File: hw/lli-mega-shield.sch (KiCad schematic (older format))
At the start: 6 parts

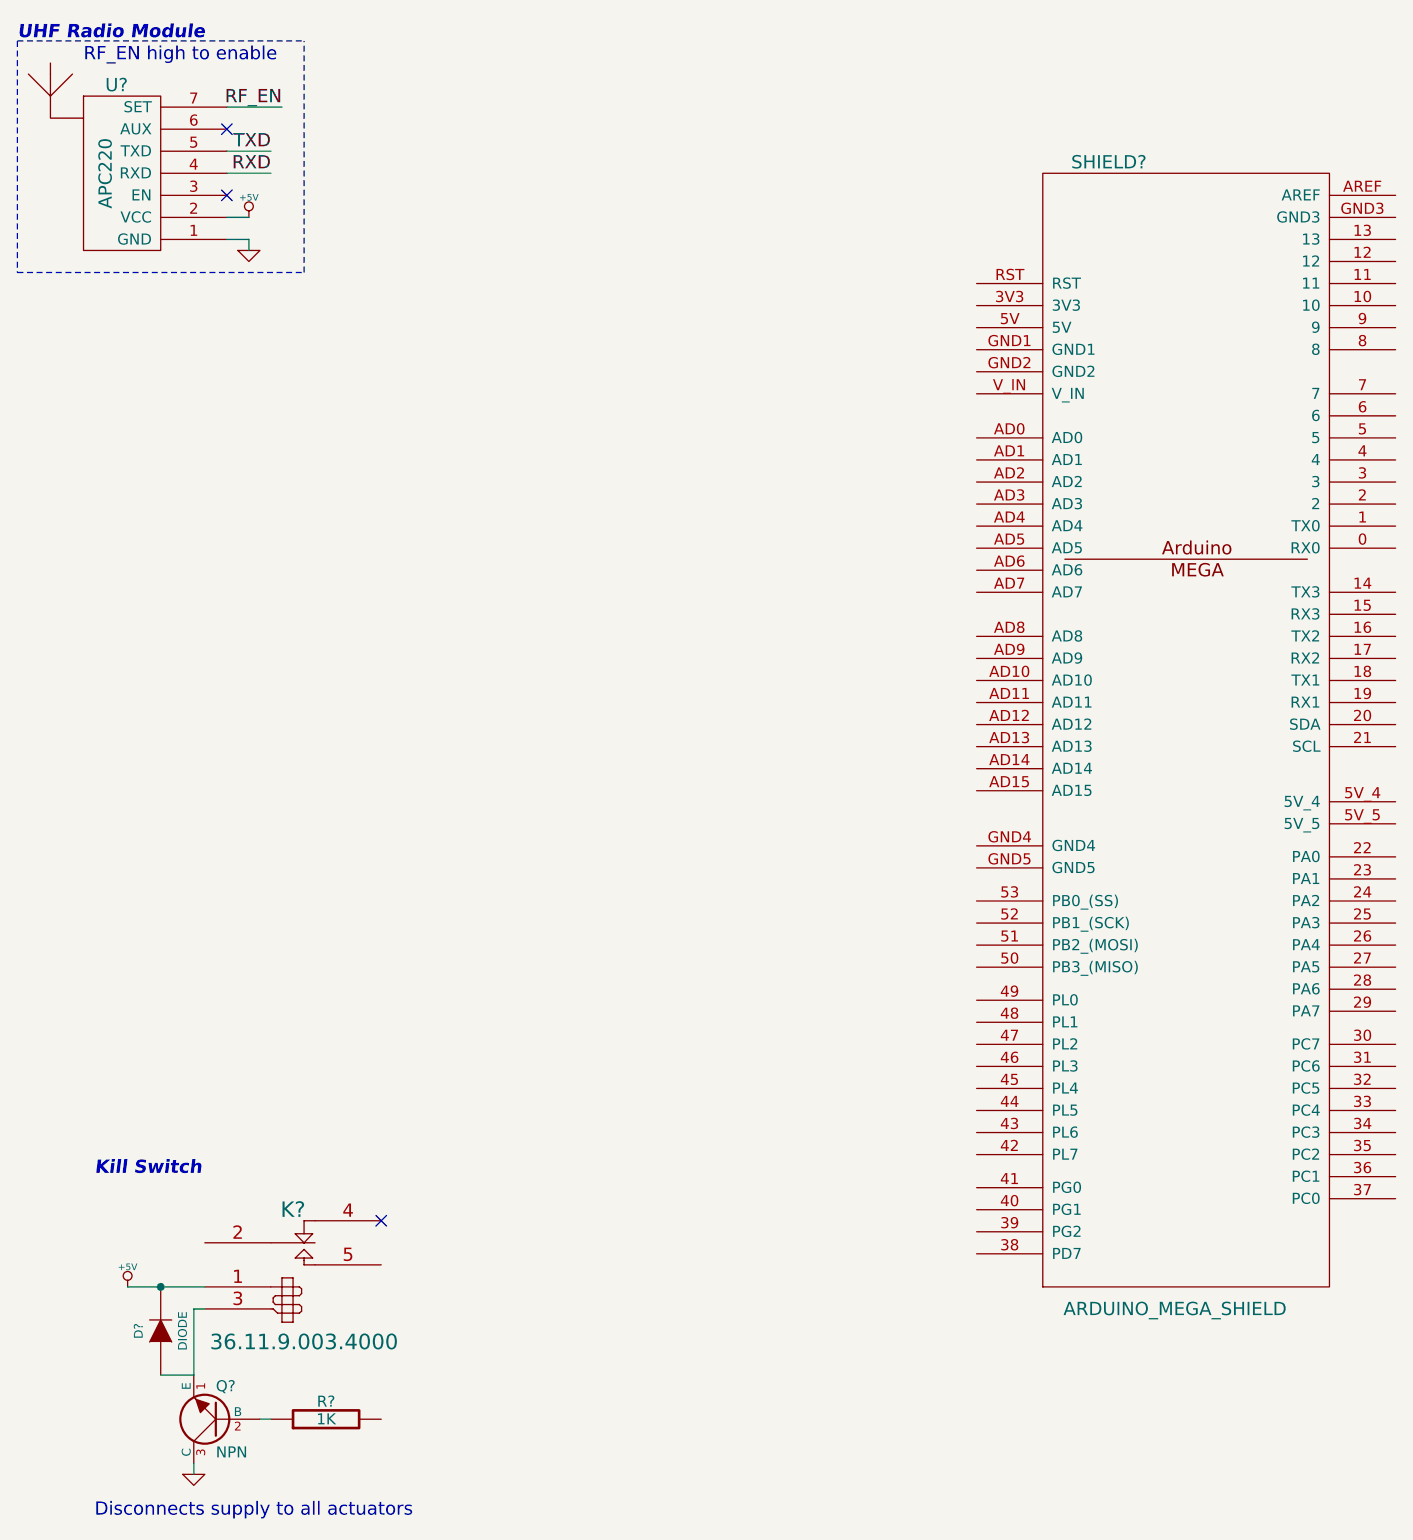
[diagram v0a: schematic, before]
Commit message: Some schematics
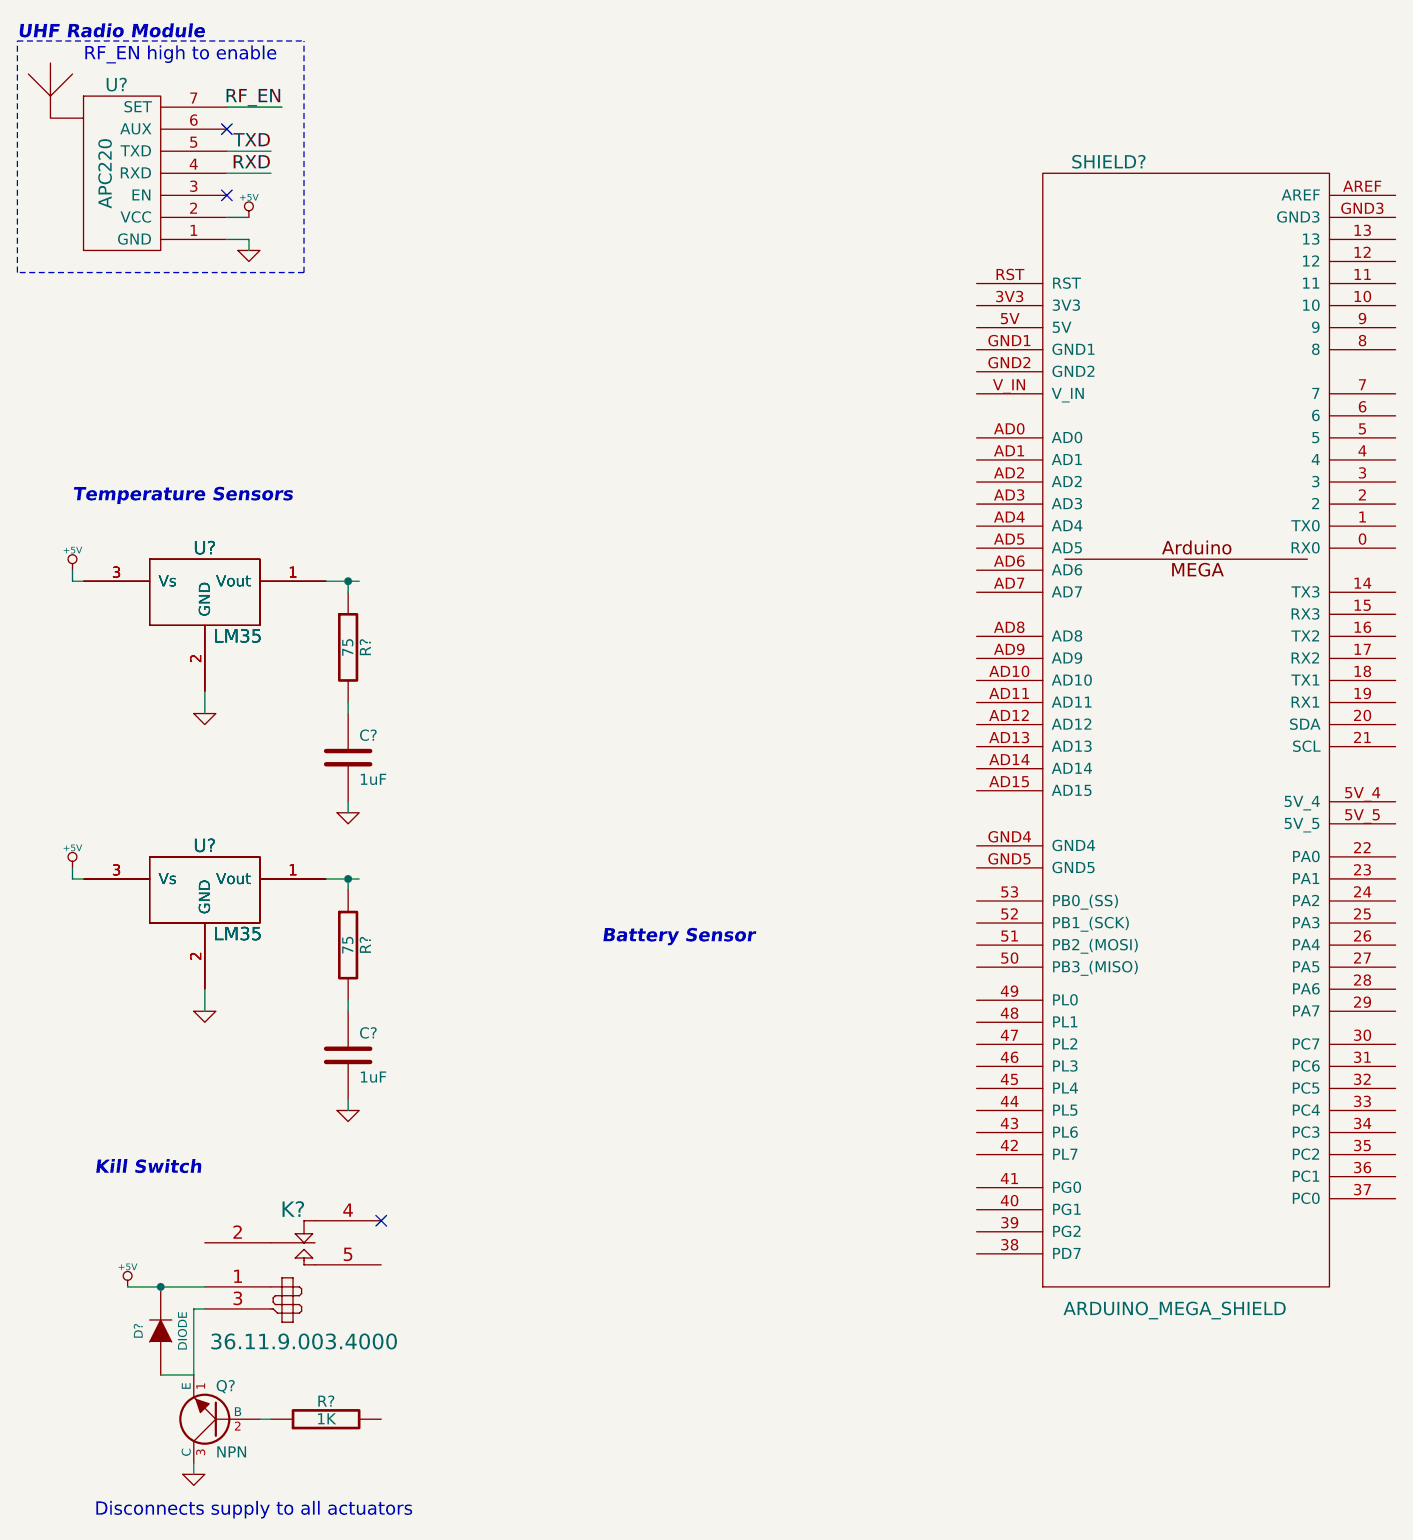
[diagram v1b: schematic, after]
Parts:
- added C? (x2): 1uF, symbol C
- added R? (x2): 75, symbol R
- added U? (x4): LM35, symbol LM35
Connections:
- wire segments 12 -> 26
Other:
- note added: "Battery Sensor"
- note added: "Temperature Sensors"
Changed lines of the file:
@@
-EESchema Schematic File Version 2  date fre 07 sep 2012 19:08:03 CEST
+EESchema Schematic File Version 2  date fre 07 sep 2012 20:49:57 CEST
 LIBS:power
 LIBS:device
@@
 Comment4 ""
 $EndDescr
+Text Notes 3300 4800 0    60   Italic 12
+Battery Sensor
+Text Notes 900  2800 0    60   Italic 12
+Temperature Sensors
+$Comp
+L LM35 U?
+U 1 1 504A41AE
+P 1500 4500
+F 0 "U?" H 1500 4650 60  0000 C CNN
+F 1 "LM35" H 1650 4250 60  0000 C CNN
+	1    1500 4500
+	1    0    0    -1
+$EndComp
+$Comp
+L R R?
+U 1 1 504A41AD
+P 2150 4800
+F 0 "R?" V 2230 4800 50  0000 C CNN
+F 1 "75" V 2150 4800 50  0000 C CNN
+	1    2150 4800
+	1    0    0    -1
+$EndComp
+$Comp
+L C C?
+U 1 1 504A41AC
+P 2150 5300
+F 0 "C?" H 2200 5400 50  0000 L CNN
+F 1 "1uF" H 2200 5200 50  0000 L CNN
+	1    2150 5300
+	1    0    0    -1
+$EndComp
+$Comp
+L GND #PWR?
+U 1 1 504A41AB
+P 1500 5100
+F 0 "#PWR?" H 1500 5100 30  0001 C CNN
+F 1 "GND" H 1500 5030 30  0001 C CNN
+	1    1500 5100
+	1    0    0    -1
+$EndComp
+$Comp
+L +5V #PWR?
+U 1 1 504A41AA
+P 900 4450
+F 0 "#PWR?" H 900 4540 20  0001 C CNN
+F 1 "+5V" H 900 4540 30  0000 C CNN
+	1    900  4450
+	1    0    0    -1
+$EndComp
+$Comp
+L LM35 U?
+U 1 1 504A41A9
+P 1500 4500
+F 0 "U?" H 1500 4650 60  0000 C CNN
+F 1 "LM35" H 1650 4250 60  0000 C CNN
+	1    1500 4500
+	1    0    0    -1
+$EndComp
+$Comp
+L GND #PWR?
+U 1 1 504A41A8
+P 2150 5550
+F 0 "#PWR?" H 2150 5550 30  0001 C CNN
+F 1 "GND" H 2150 5480 30  0001 C CNN
+	1    2150 5550
+	1    0    0    -1
+$EndComp
+Wire Wire Line
+	900  4500 950  4500
+Wire Wire Line
+	900  4450 900  4500
+Wire Wire Line
+	2200 4500 2050 4500
+Wire Wire Line
+	2150 5100 2150 5050
+Wire Wire Line
+	2150 4500 2150 4550
+Connection ~ 2150 4500
+Wire Wire Line
+	1500 5100 1500 5000
+Wire Wire Line
+	2150 5550 2150 5500
+Wire Wire Line
+	2150 4200 2150 4150
+Wire Wire Line
+	1500 3750 1500 3650
+Connection ~ 2150 3150
+Wire Wire Line
+	2150 3150 2150 3200
+Wire Wire Line
+	2150 3750 2150 3700
+Wire Wire Line
+	1450 7200 1450 7150
+Wire Wire Line
+	1450 6450 1450 6750
+Wire Wire Line
+	1450 6450 1500 6450
+Wire Wire Line
+	1850 1000 1600 1000
+Wire Wire Line
+	1800 1300 1600 1300
+Wire Wire Line
+	1600 1600 1700 1600
+Wire Wire Line
+	1700 1600 1700 1650
+Wire Wire Line
+	1600 1500 1700 1500
+Wire Wire Line
+	1600 1200 1800 1200
+Wire Notes Line
+	1950 1750 1950 700
+Wire Notes Line
+	1950 1750 650  1750
+Wire Notes Line
+	650  1750 650  700
+Wire Notes Line
+	650  700  1950 700
+Wire Wire Line
+	1150 6350 1500 6350
+Connection ~ 1300 6350
+Wire Wire Line
+	1450 6750 1300 6750
+Wire Wire Line
+	1750 6950 1800 6950
+Wire Wire Line
+	2200 3150 2050 3150
+Wire Wire Line
+	900  3100 900  3150
+Wire Wire Line
+	900  3150 950  3150
+$Comp
+L GND #PWR?
+U 1 1 504A414B
+P 2150 4200
+F 0 "#PWR?" H 2150 4200 30  0001 C CNN
+F 1 "GND" H 2150 4130 30  0001 C CNN
+	1    2150 4200
+	1    0    0    -1
+$EndComp
+$Comp
+L LM35 U?
+U 1 1 504A39E8
+P 1500 3150
+F 0 "U?" H 1500 3300 60  0000 C CNN
+F 1 "LM35" H 1650 2900 60  0000 C CNN
+	1    1500 3150
+	1    0    0    -1
+$EndComp
+$Comp
+L +5V #PWR?
+U 1 1 504A39DE
+P 900 3100
+F 0 "#PWR?" H 900 3190 20  0001 C CNN
+F 1 "+5V" H 900 3190 30  0000 C CNN
+	1    900  3100
+	1    0    0    -1
+$EndComp
+$Comp
+L GND #PWR?
+U 1 1 504A39D5
+P 1500 3750
+F 0 "#PWR?" H 1500 3750 30  0001 C CNN
+F 1 "GND" H 1500 3680 30  0001 C CNN
+	1    1500 3750
+	1    0    0    -1
+$EndComp
+$Comp
+L C C?
+U 1 1 504A39C7
+P 2150 3950
+F 0 "C?" H 2200 4050 50  0000 L CNN
+F 1 "1uF" H 2200 3850 50  0000 L CNN
+	1    2150 3950
+	1    0    0    -1
+$EndComp
+$Comp
+L R R?
+U 1 1 504A39C1
+P 2150 3450
+F 0 "R?" V 2230 3450 50  0000 C CNN
+F 1 "75" V 2150 3450 50  0000 C CNN
+	1    2150 3450
+	1    0    0    -1
+$EndComp
+$Comp
+L LM35 U?
+U 1 1 504A39B9
+P 1500 3150
+F 0 "U?" H 1500 3300 60  0000 C CNN
+F 1 "LM35" H 1650 2900 60  0000 C CNN
+	1    1500 3150
+	1    0    0    -1
+$EndComp
 Text Notes 1000 7400 0    60   ~ 0
 Disconnects supply to all actuators
@@
 $EndComp
 NoConn ~ 2300 6050
-Wire Wire Line
-	1750 6950 1800 6950
-Wire Wire Line
-	1300 6750 1450 6750
-Connection ~ 1300 6350
-Wire Wire Line
-	1150 6350 1500 6350
-Wire Notes Line
-	650  700  1950 700
-Wire Notes Line
-	650  700  650  1750
-Wire Notes Line
-	650  1750 1950 1750
-Wire Notes Line
-	1950 1750 1950 700
-Wire Wire Line
-	1600 1200 1800 1200
-Wire Wire Line
-	1600 1500 1700 1500
-Wire Wire Line
-	1700 1650 1700 1600
-Wire Wire Line
-	1700 1600 1600 1600
-Wire Wire Line
-	1800 1300 1600 1300
-Wire Wire Line
-	1850 1000 1600 1000
-Wire Wire Line
-	1500 6450 1450 6450
-Wire Wire Line
-	1450 6450 1450 6750
-Wire Wire Line
-	1450 7200 1450 7150
 $Comp
 L R R?
